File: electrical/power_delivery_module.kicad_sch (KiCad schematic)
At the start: 9 parts, among them J2 Screw_Terminal_01x01, U4 UA78L05AI

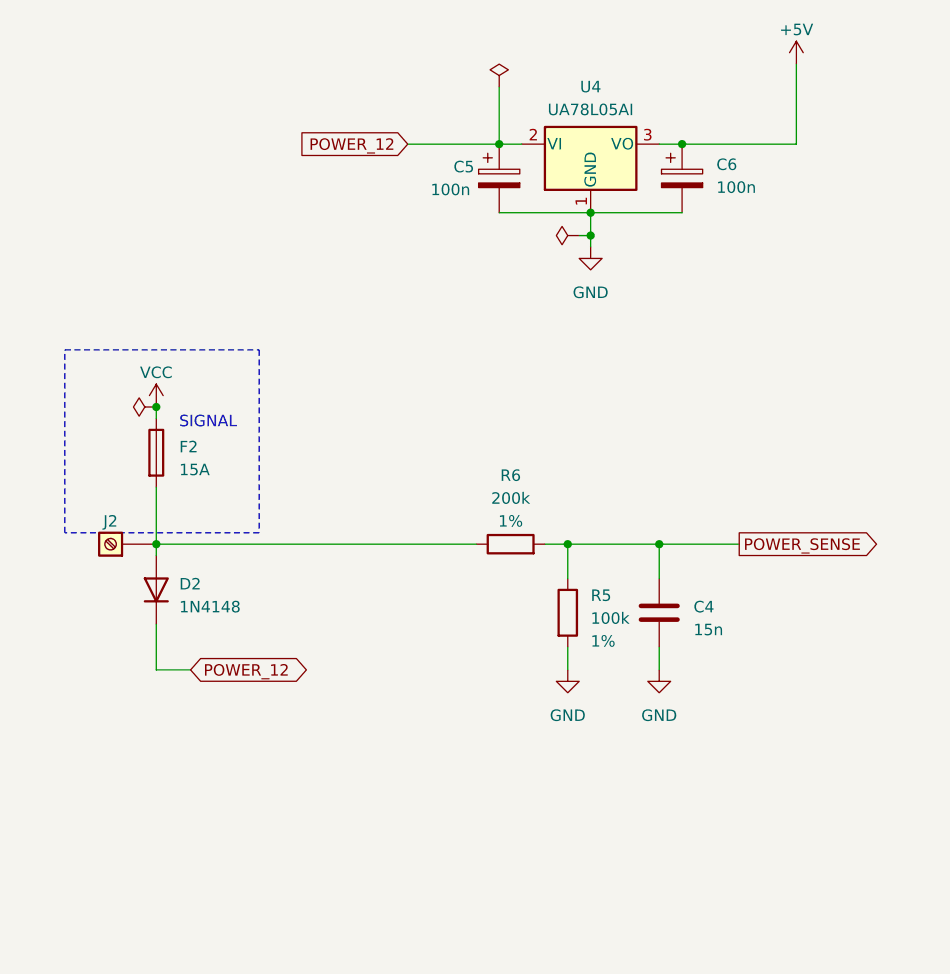
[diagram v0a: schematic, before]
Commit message: Względenie działa
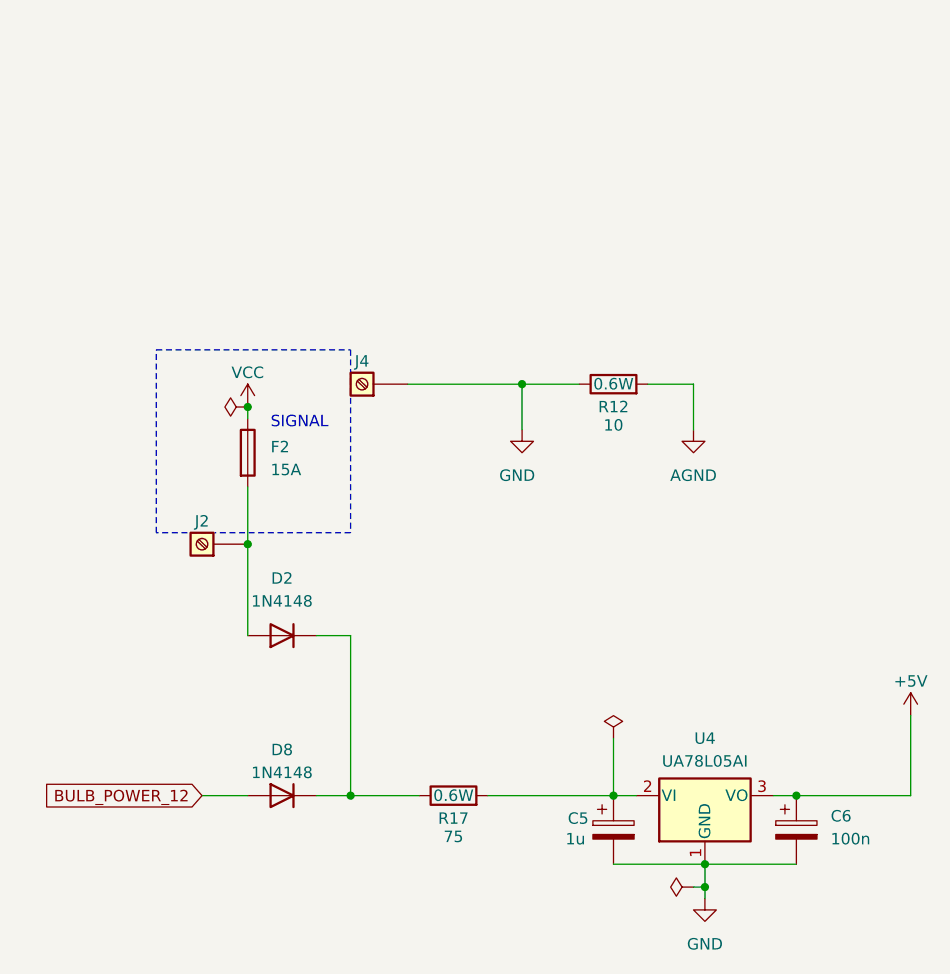
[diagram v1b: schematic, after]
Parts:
- removed C4: 15n, symbol Device:C
- removed R5: 100k, symbol Device:R
- removed R6: 200k, symbol Device:R
- added D8: 1N4148, Diode_THT:D_DO-41_SOD81_P10.16mm_Horizontal, symbol Diode:1N4002
- added J4: Screw_Terminal_01x01, symbol Connector:Screw_Terminal_01x01
- added R12: 10, symbol Device:R
- added R17: 75, symbol Device:R
- C5: value 100n -> 1u
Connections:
- net GND: now also J4.1 (Pin_1), R12.1
- net POWER_12: no longer names the net of C5.1, U4.2 (VI)
- net POWER_12: now also R17.2; no longer D2.1 (K)
- new net: D2.1 (K), D8.1 (K), R17.1
- new net AGND: R12.2
- new net BULB_POWER_12: D8.2 (A)
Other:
- moved on the sheet: C5, C6, D2, F2, J2, U4
